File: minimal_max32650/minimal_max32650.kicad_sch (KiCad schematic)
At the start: 105 parts, among them J1 FTSH-105-01-L-DV-K, J2 CLP-150-02-G-D-BE, Q1 50 V, Q2 50 V, U1 MX25U6432FZNI02, U2 MAXQ1065GTC+, U3 ADT75BRMZ, U4 MAX32650GCE+, U5 S80KS5122GABHM020, U6 ADP225ACPZ-R7

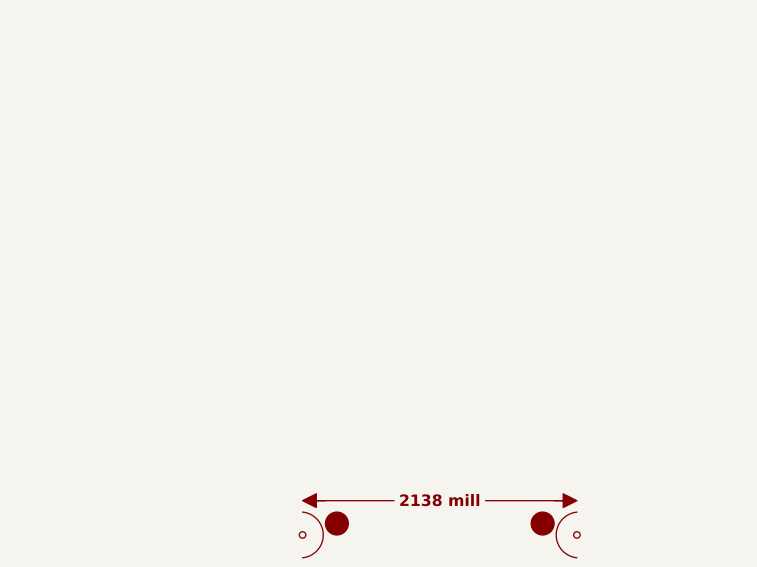
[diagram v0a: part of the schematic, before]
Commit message: test workflow render
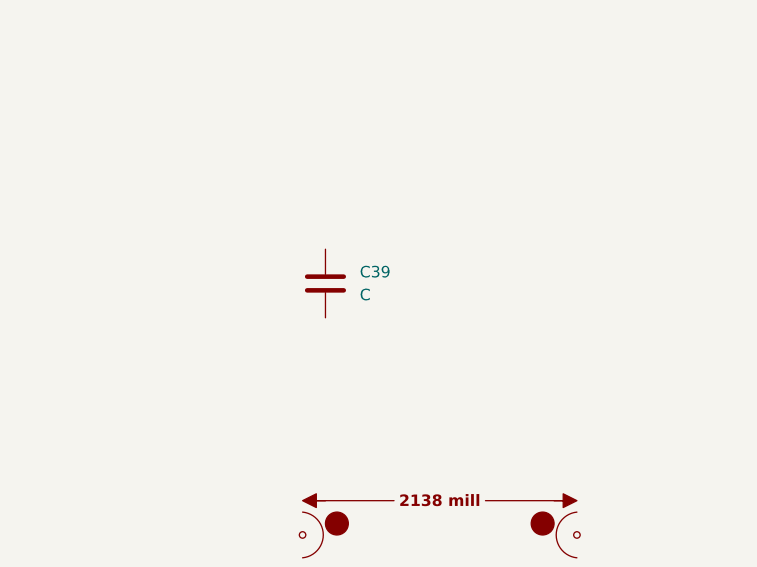
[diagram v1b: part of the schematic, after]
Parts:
- added C39: C, Capacitor_SMD:C_0805_2012Metric, symbol Device:C
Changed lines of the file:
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@@
+	)
+	(symbol
+		(lib_id "Device:C")
+		(at 63.5 142.24 0)
+		(unit 1)
+		(exclude_from_sim no)
+		(in_bom yes)
+		(on_board yes)
+		(dnp no)
+		(fields_autoplaced yes)
+		(property "Reference" "C39"
+			(at 67.31 140.9699 0)
+			(effects
+				(font
+					(size 1.27 1.27)
+				)
+				(justify left)
+			)
+		)
+		(property "Value" "C"
+			(at 67.31 143.5099 0)
+			(effects
+				(font
+					(size 1.27 1.27)
+				)
+				(justify left)
+			)
+		)
+		(property "Footprint" "Capacitor_SMD:C_0805_2012Metric"
+			(at 64.4652 146.05 0)
+			(effects
+				(font
+					(size 1.27 1.27)
+				)
+				(hide yes)
+			)
+		)
+		(property "Datasheet" "~"
+			(at 63.5 142.24 0)
+			(effects
+				(font
+					(size 1.27 1.27)
+				)
+				(hide yes)
+			)
+		)
+		(property "Description" "Unpolarized capacitor"
+			(at 63.5 142.24 0)
+			(effects
+				(font
+					(size 1.27 1.27)
+				)
+				(hide yes)
+			)
+		)
+		(pin "1"
+		)
+		(pin "2"
+		)
+		(instances
+			(project ""
+				(path "/95623a5c-6e9d-4c1c-be90-b39230c07c79"
+					(reference "C39")
+					(unit 1)
+				)
+			)
+		)
 	)
 	(symbol

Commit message: test workflow render 2
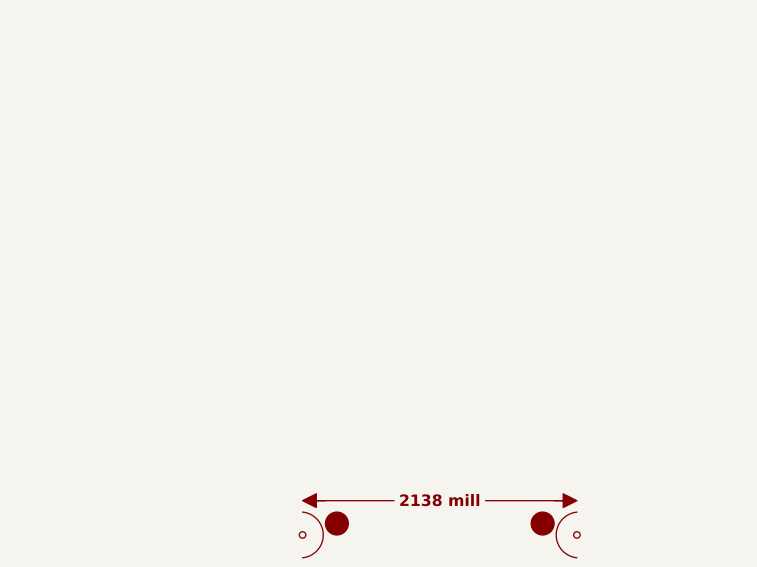
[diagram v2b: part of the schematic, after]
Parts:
- removed C39: C, Capacitor_SMD:C_0805_2012Metric, symbol Device:C
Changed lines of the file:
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@@
-	)
-	(symbol
-		(lib_id "Device:C")
-		(at 63.5 142.24 0)
-		(unit 1)
-		(exclude_from_sim no)
-		(in_bom yes)
-		(on_board yes)
-		(dnp no)
-		(fields_autoplaced yes)
-		(property "Reference" "C39"
-			(at 67.31 140.9699 0)
-			(effects
-				(font
-					(size 1.27 1.27)
-				)
-				(justify left)
-			)
-		)
-		(property "Value" "C"
-			(at 67.31 143.5099 0)
-			(effects
-				(font
-					(size 1.27 1.27)
-				)
-				(justify left)
-			)
-		)
-		(property "Footprint" "Capacitor_SMD:C_0805_2012Metric"
-			(at 64.4652 146.05 0)
-			(effects
-				(font
-					(size 1.27 1.27)
-				)
-				(hide yes)
-			)
-		)
-		(property "Datasheet" "~"
-			(at 63.5 142.24 0)
-			(effects
-				(font
-					(size 1.27 1.27)
-				)
-				(hide yes)
-			)
-		)
-		(property "Description" "Unpolarized capacitor"
-			(at 63.5 142.24 0)
-			(effects
-				(font
-					(size 1.27 1.27)
-				)
-				(hide yes)
-			)
-		)
-		(pin "1"
-		)
-		(pin "2"
-		)
-		(instances
-			(project ""
-				(path "/95623a5c-6e9d-4c1c-be90-b39230c07c79"
-					(reference "C39")
-					(unit 1)
-				)
-			)
-		)
 	)
 	(symbol
